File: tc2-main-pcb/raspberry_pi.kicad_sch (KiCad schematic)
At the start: 21 parts, among them J1 Screw_Terminal_01x01, J2 Screw_Terminal_01x01, J4 Raspberry_Pi_2_3, J5 Screw_Terminal_01x01, J6 Screw_Terminal_01x01, J8 Screw_Terminal_01x01, U14 MAX98357AEWL+T, U15 74HC4052, U17 PCA9515ADP,118

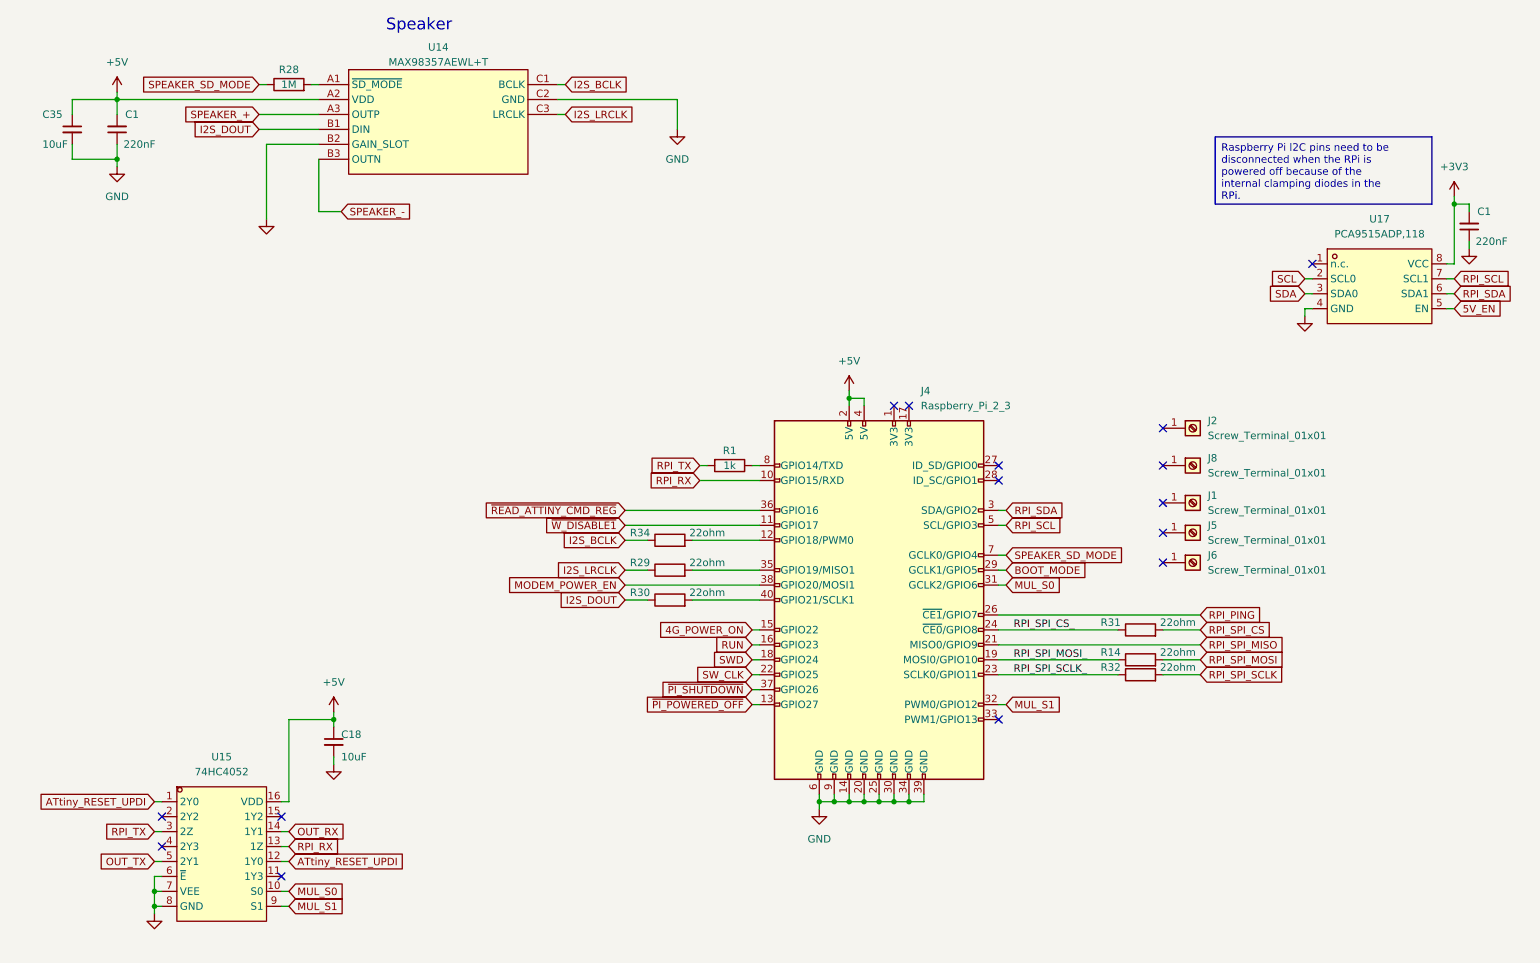
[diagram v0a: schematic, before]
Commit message: v0.4.0
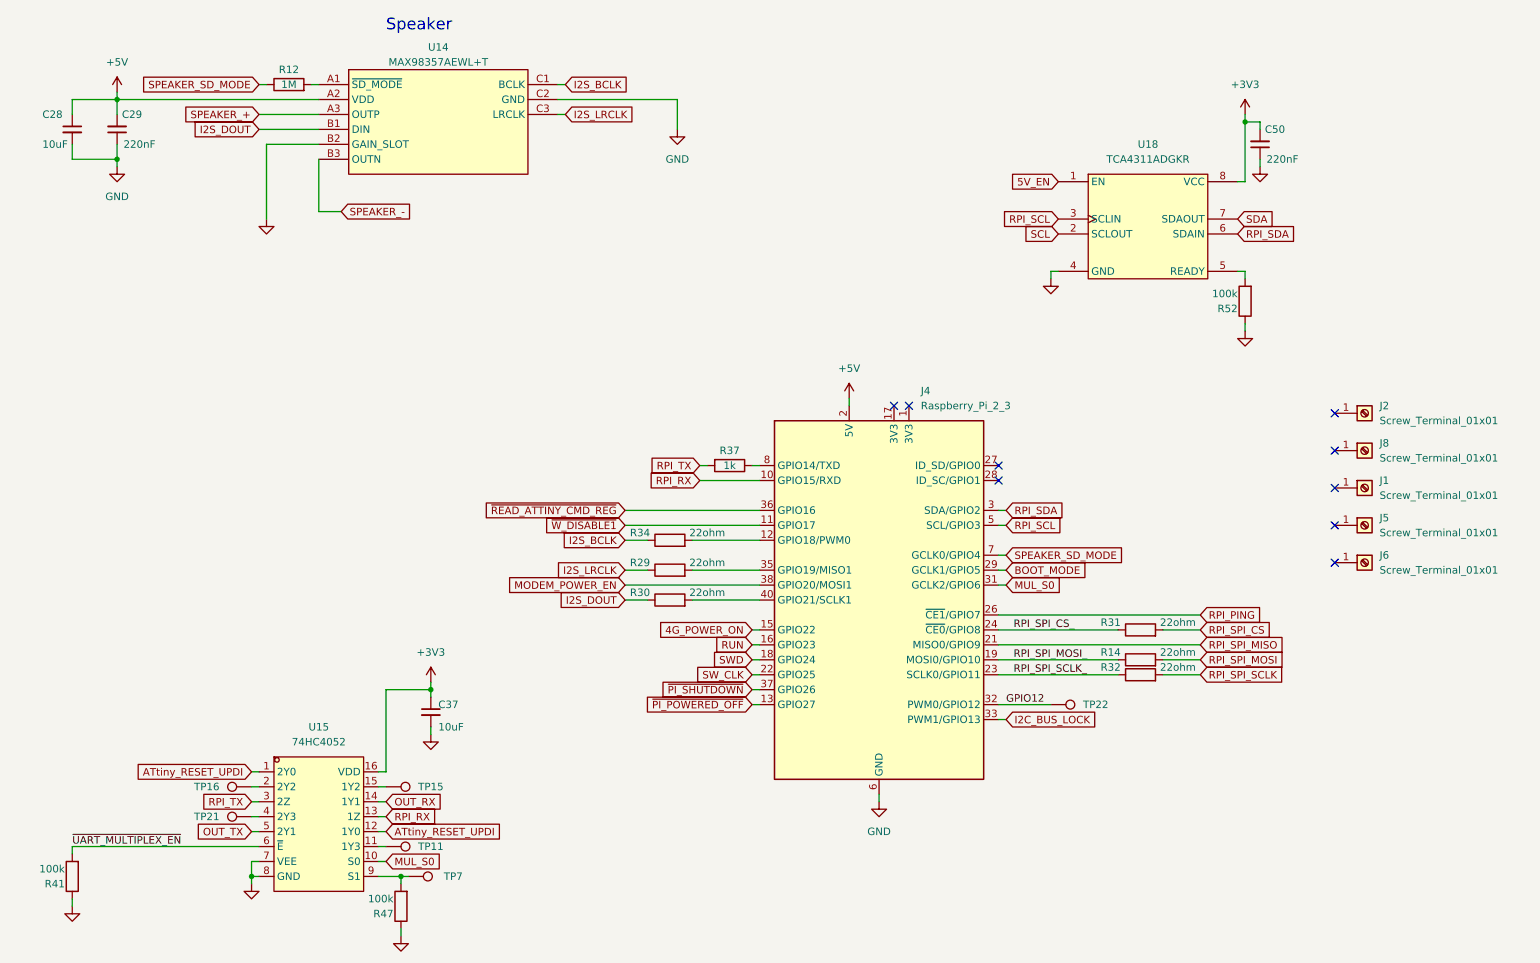
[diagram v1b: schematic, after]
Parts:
- removed U17: PCA9515ADP,118, Package_SO:TSSOP-8_3x3mm_P0.65mm, symbol cacophony-library:PCA9515ADP,118
- added R41, R47, R52: 100k, Resistor_SMD:R_0402_1005Metric, symbol Device:R
- added TP11, TP15, TP16, TP21, TP22, TP7: TestPoint, cacophony-library:TP, symbol Connector:TestPoint
- added U18: TCA4311ADGKR, Package_SO:MSOP-8_3x3mm_P0.65mm, symbol cacophony-library:TCA4311ADGKR
- J1, J2, J5, J6, J8: footprint cacophony-library:SMTSO25 -> cacophony-library:smd_nut_SMTSO25
- J4: symbol Connector:Raspberry_Pi_2_3 -> cacophony-library:Raspberry_Pi_2_3
- U14: LCSC (none) -> C2682619; LCSC Part C2682619 -> (none)
- U15: LCSC (none) -> C111594; LCSC Part C111594 -> (none)
- renumbered C35 to C28, C1 to C29, C18 to C37, C1 to C50, R28 to R12, R1 to R37
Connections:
- net +3V3: now also C37.1, U15.16 (VDD), U18.8 (VCC)
- net +5V: no longer C37.1, U15.16 (VDD)
- net 5V_EN: now also U18.1 (EN)
- net GND: now also R41.1, R47.1, R52.1, U18.4 (GND); no longer U15.6 (~{E})
- net RPI_SCL: now also U18.3 (SCLIN)
- net RPI_SDA: now also U18.6 (SDAIN)
- net SCL: now also U18.2 (SCLOUT)
- net SDA: now also U18.7 (SDAOUT)
- net I2C_BUS_LOCK: now reaches J4.33 (PWM1/GPIO13)
- net at U15.11 (1Y3): now also TP11.1
- net at U15.15 (1Y2): now also TP15.1
- net at U15.2 (2Y2): now also TP16.1
- net at U15.4 (2Y3): now also TP21.1
- net MUL_S1: no longer names the net of U15.9 (S1)
- net MUL_S1: now also R47.2, TP7.1; no longer J4.32 (PWM0/GPIO12)
- new net: R52.2, U18.5 (READY)
- new net GPIO12: J4.32 (PWM0/GPIO12), TP22.1
- new net ~{UART_MULTIPLEX_EN}: R41.2, U15.6 (~{E})
- no-connect marks 15 -> 9
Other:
- moved on the sheet: C37, C50, J1, J2, J5, J6, J8, U15
